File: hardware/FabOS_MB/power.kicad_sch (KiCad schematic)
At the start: 22 parts, among them U1 TPS563201, U2 TDPOWER TAS12-5-W2

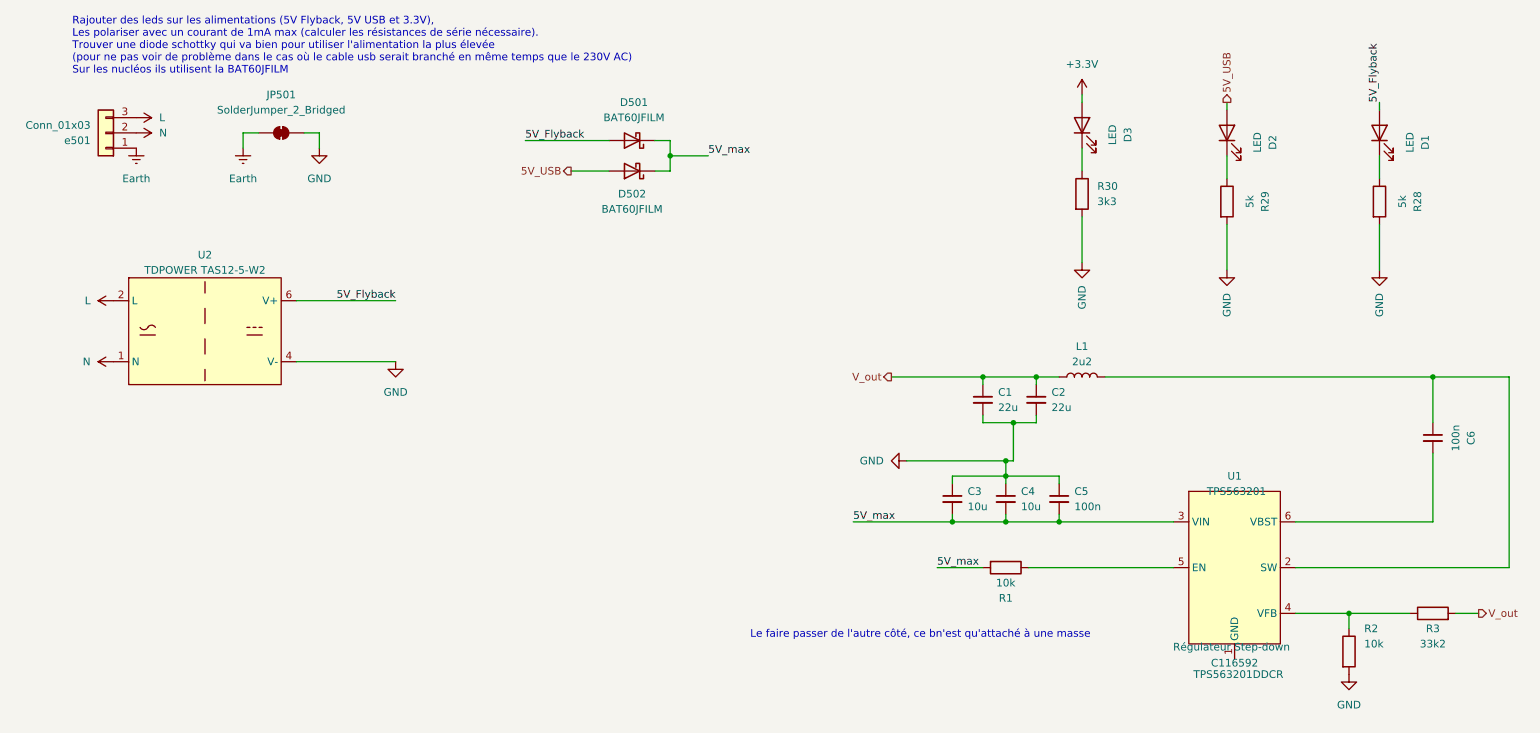
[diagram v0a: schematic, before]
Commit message: update pcb
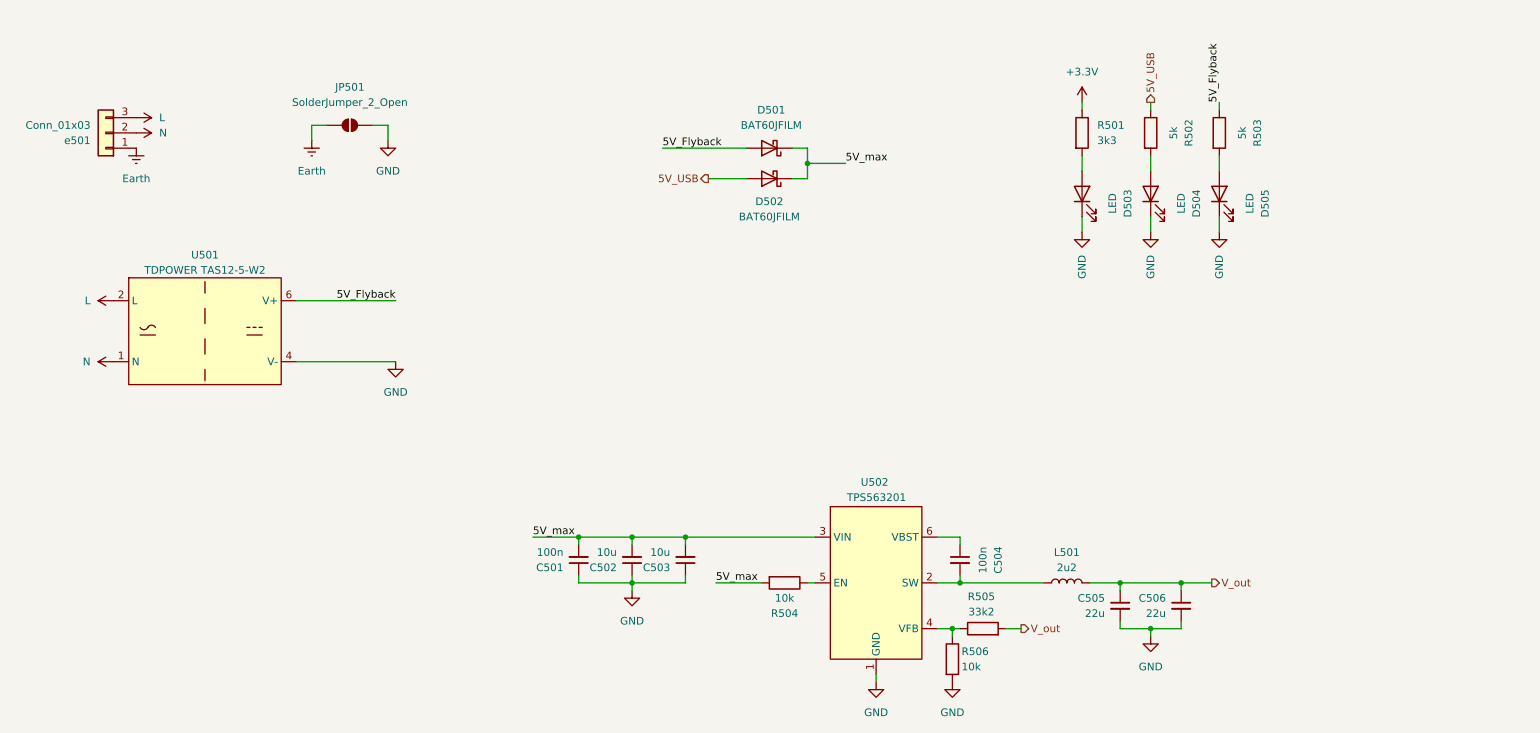
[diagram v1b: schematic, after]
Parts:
- removed C1, C2: 22u, symbol Device:C_Small
- removed D1, D2, D3: LED, symbol Device:LED
- removed JP501: SolderJumper_2_Bridged, symbol Jumper:SolderJumper_2_Bridged
- removed L1: 2u2, symbol Device:L
- removed R28, R29: 5k, symbol Device:R
- removed R30: 3k3, symbol Device:R
- added C505, C506: 22u, symbol Device:C_Small
- added D503, D504, D505: LED, symbol Device:LED
- added JP501: SolderJumper_2_Open, symbol Jumper:SolderJumper_2_Open
- added L501: 2u2, symbol Device:L
- added R501: 3k3, symbol Device:R
- added R502, R503: 5k, symbol Device:R
- renumbered C5 to C501, C4 to C502, C3 to C503, C6 to C504, R1 to R504, R3 to R505, R2 to R506, U2 to U501, U1 to U502
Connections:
- net 5V_Flyback: now also R503.1
- net 5V_USB: now also R502.1
- net Earth: now also JP501.1 (A)
- net GND: now also U502.1 (GND), C505.2, C506.2, D503.1 (K), D504.1 (K), D505.1 (K), JP501.2 (B)
- net V_out: now also C505.1, C506.1, L501.1
- net at U502.2 (SW): now also C504.2, L501.2; no longer C504.1
- net at U502.6 (VBST): now also C504.1; no longer C504.2
- new net: D505.2 (A), R503.2
- new net: D504.2 (A), R502.2
- new net: D503.2 (A), R501.2
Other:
- note removed: "Le faire passer de l'autre côté, ce bn'est qu'attaché à une masse"
- note removed: "Rajouter des leds sur les alimentations (5V Flyback, 5V USB et 3.3V), Les polariser avec un courant de 1mA max (calculer les résistances de série nécessaire). Trouver une diode schottky qui va bien pour utiliser l'alimentation la plus élevée (pour ne pas voir de problème dans le cas où le cable usb serait branché en même temps que le 230V AC) Sur les nucléos ils utilisent la BAT60JFILM"
- moved on the sheet: C501, C502, C503, C504, D501, D502, R504, R505, R506, U502

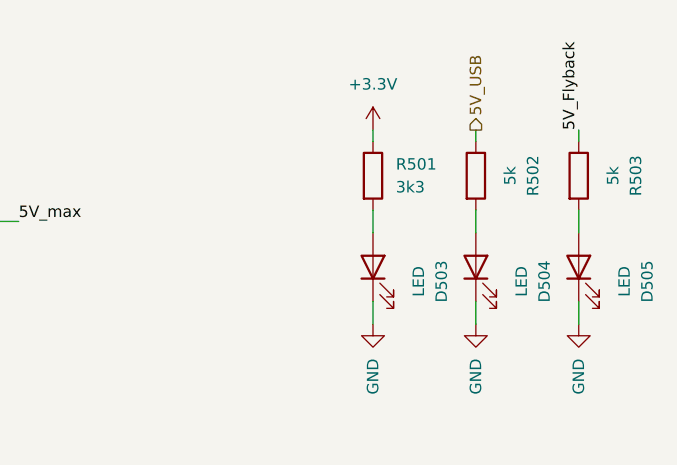
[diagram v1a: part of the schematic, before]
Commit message: update
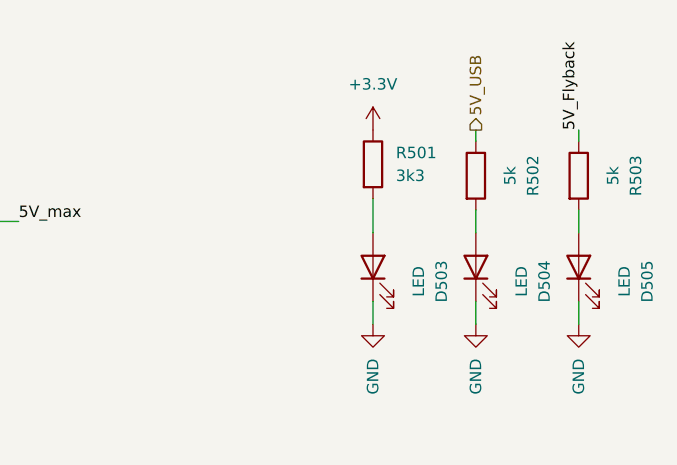
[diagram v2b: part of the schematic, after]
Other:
- moved on the sheet: R501
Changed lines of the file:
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@@
 	(wire
 		(pts
-			(xy 204.47 44.45) (xy 204.47 41.91)
+			(xy 204.47 44.45) (xy 204.47 40.64)
 		)
 		(stroke
@@
 		(pts
 			(xy 120.65 106.68) (xy 120.65 105.41)
-		)
-		(stroke
-			(width 0)
-			(type default)
-		)
-	)
-	(wire
-		(pts
-			(xy 204.47 34.29) (xy 204.47 33.02)
 		)
 		(stroke
@@
 	(symbol
 		(lib_id "Device:R")
-		(at 204.47 38.1 0)
+		(at 204.47 36.83 0)
 		(unit 1)
 		(exclude_from_sim no)
@@
 		(fields_autoplaced yes)
 		(property "Reference" "R501"
-			(at 207.01 36.8299 0)
+			(at 207.01 35.5599 0)
 			(effects
 				(font
@@
 		)
 		(property "Value" "3k3"
-			(at 207.01 39.3699 0)
+			(at 207.01 38.0999 0)
 			(effects
 				(font
@@
 		)
 		(property "Footprint" ""
-			(at 202.692 38.1 90)
+			(at 202.692 36.83 90)
 			(effects
 				(font
@@
 		)
 		(property "Datasheet" "~"
-			(at 204.47 38.1 0)
+			(at 204.47 36.83 0)
 			(effects
 				(font
@@
 		)
 		(property "Description" "Resistor"
-			(at 204.47 38.1 0)
-			(effects
-				(font
+			(at 204.47 36.83 0)
+			(effects
+				(font
